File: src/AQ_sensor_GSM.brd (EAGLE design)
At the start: 110 x 64 mm, 84 parts, among them IC1 MIC29302WU, IC2 MCP73831/OT, J1 F-1X03-SIP-100-32, J2 SIM8060-6-1-14-00-A, J3 PJ-002BH, Q1 MMBT2222, Q2 MMBT2222, Q3 MMBT2222, U1 LM7805S/NOPB, U2 TEXAS_INSTRUMENTS_SN74HC125TE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, U3 TEXAS_INSTRUMENTS_LM1117IMP-3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, U4 EC200UCNAB-N05-SNNSA, X1 53048-08

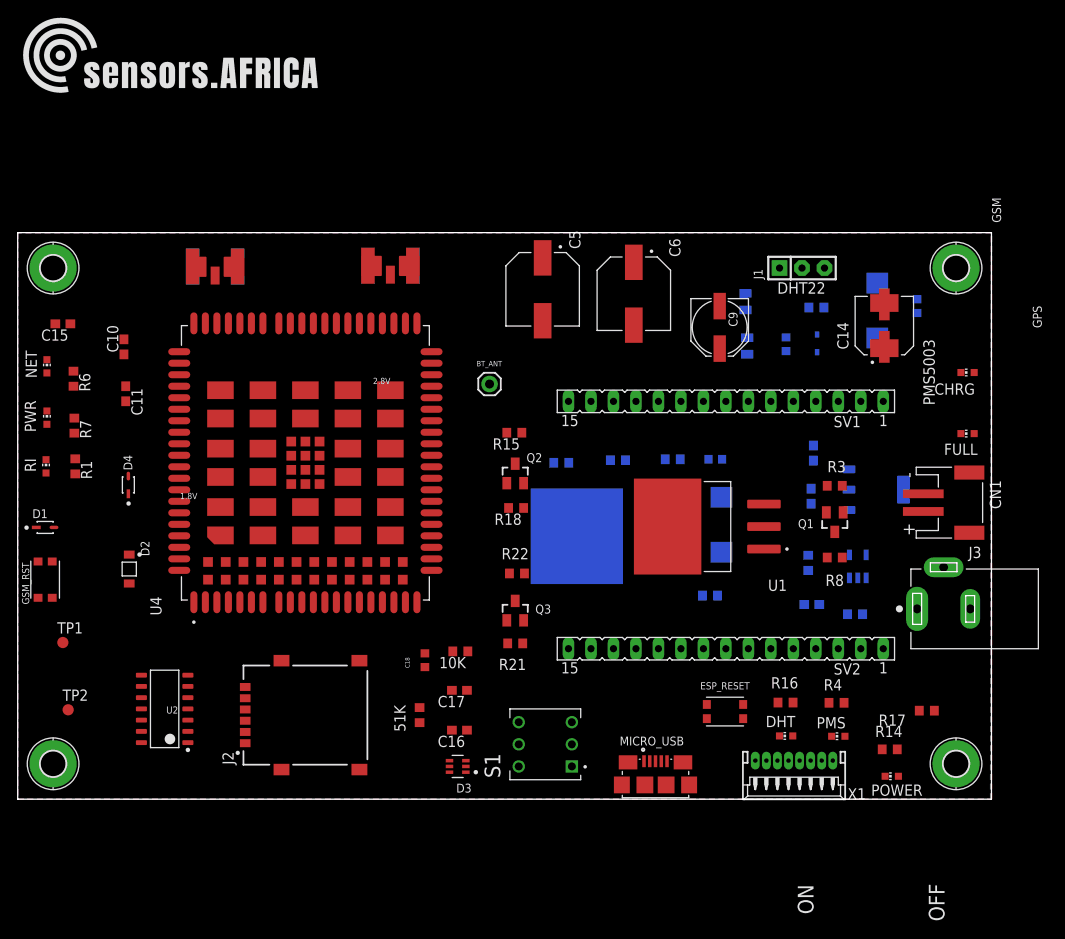
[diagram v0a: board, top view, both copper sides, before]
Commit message: PCB Routed
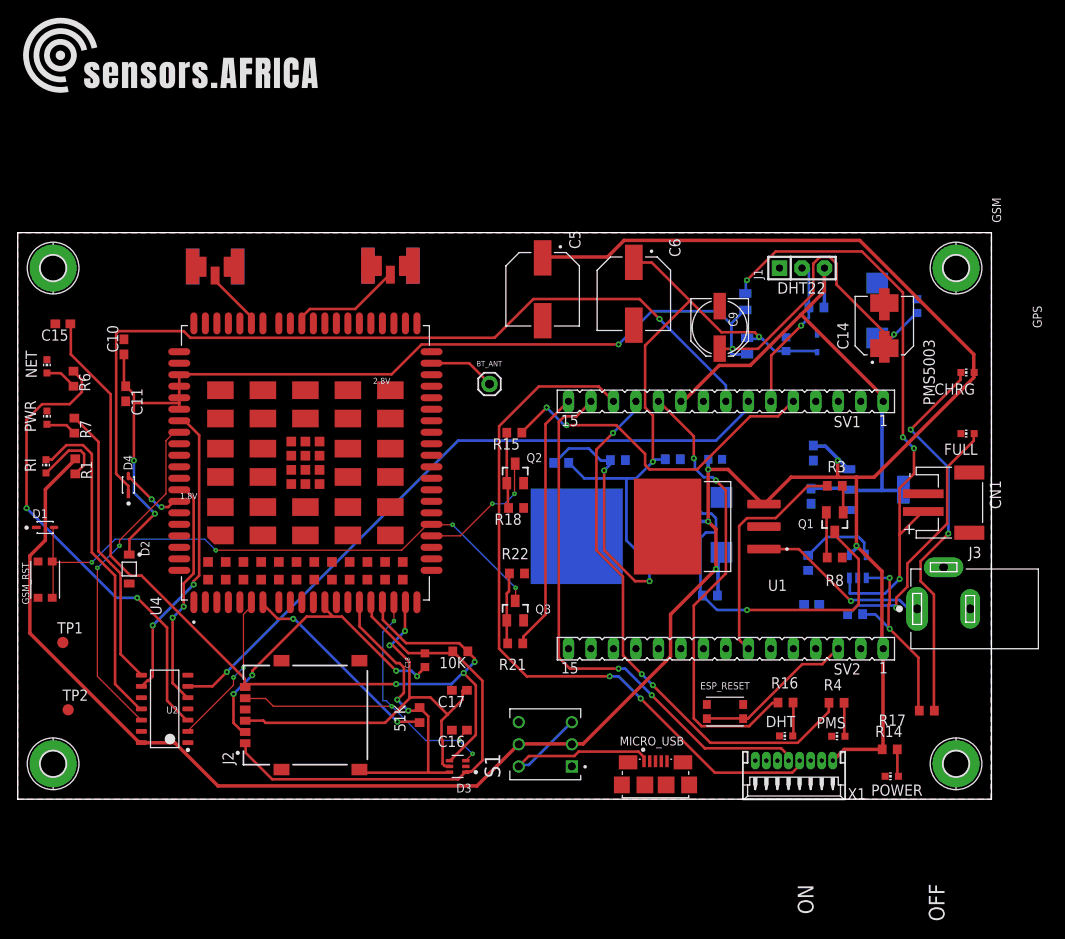
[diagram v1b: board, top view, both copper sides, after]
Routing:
- net +5V: track 0.00 -> 286.1 mm, vias 0 -> 5
- net V_LIPO: track 0.00 -> 146.3 mm, vias 0 -> 5
- net SIMDATA: track 0.00 -> 103.5 mm, vias 0 -> 3
- net GSM_RX_O: track 0.00 -> 95.6 mm, vias 0 -> 1
- net PMS_RX: track 0.00 -> 81.2 mm, vias 0 -> 2
- net GSM_TX_5V: track 0.00 -> 77.1 mm, vias 0 -> 1
- net N$34: track 0.00 -> 69.9 mm, vias 0 -> 2
- net N$39: track 0.00 -> 67.9 mm, vias 0 -> 4
- net PWRKEY: track 0.00 -> 67.8 mm, vias 0 -> 4
- net +3V3: track 0.00 -> 63.1 mm
- net PMS_TX: track 0.00 -> 62.4 mm, vias 0 -> 2
- net PMS_LED: track 0.00 -> 61.6 mm, vias 0 -> 3
- net USIM_VDD: track 0.00 -> 56.7 mm
- net NETSTAT_5V: track 0.00 -> 53.3 mm, vias 0 -> 2
- net DHT_LED: track 0.00 -> 52.1 mm, vias 0 -> 2
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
